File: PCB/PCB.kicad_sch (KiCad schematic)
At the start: 103 parts, among them J1 USB_B_Mini, J2 Screw_Terminal_01x02, J3 Conn_01x03, K1 G6K-2, Q1 IPD50R3K0CE, Q2 2N7002, SW1 SW_Omron_B3FS, U1 STM32F373C8Tx, U2 LIS3MDL, U3 INA848, U4 LM27313XMFX/NOPB, U5 OPA4189xD, U6 THS4561, U7 UCC44273, U8 REF2025AIDDCR, U9 MCP1700-3.3, Y1 8MHz

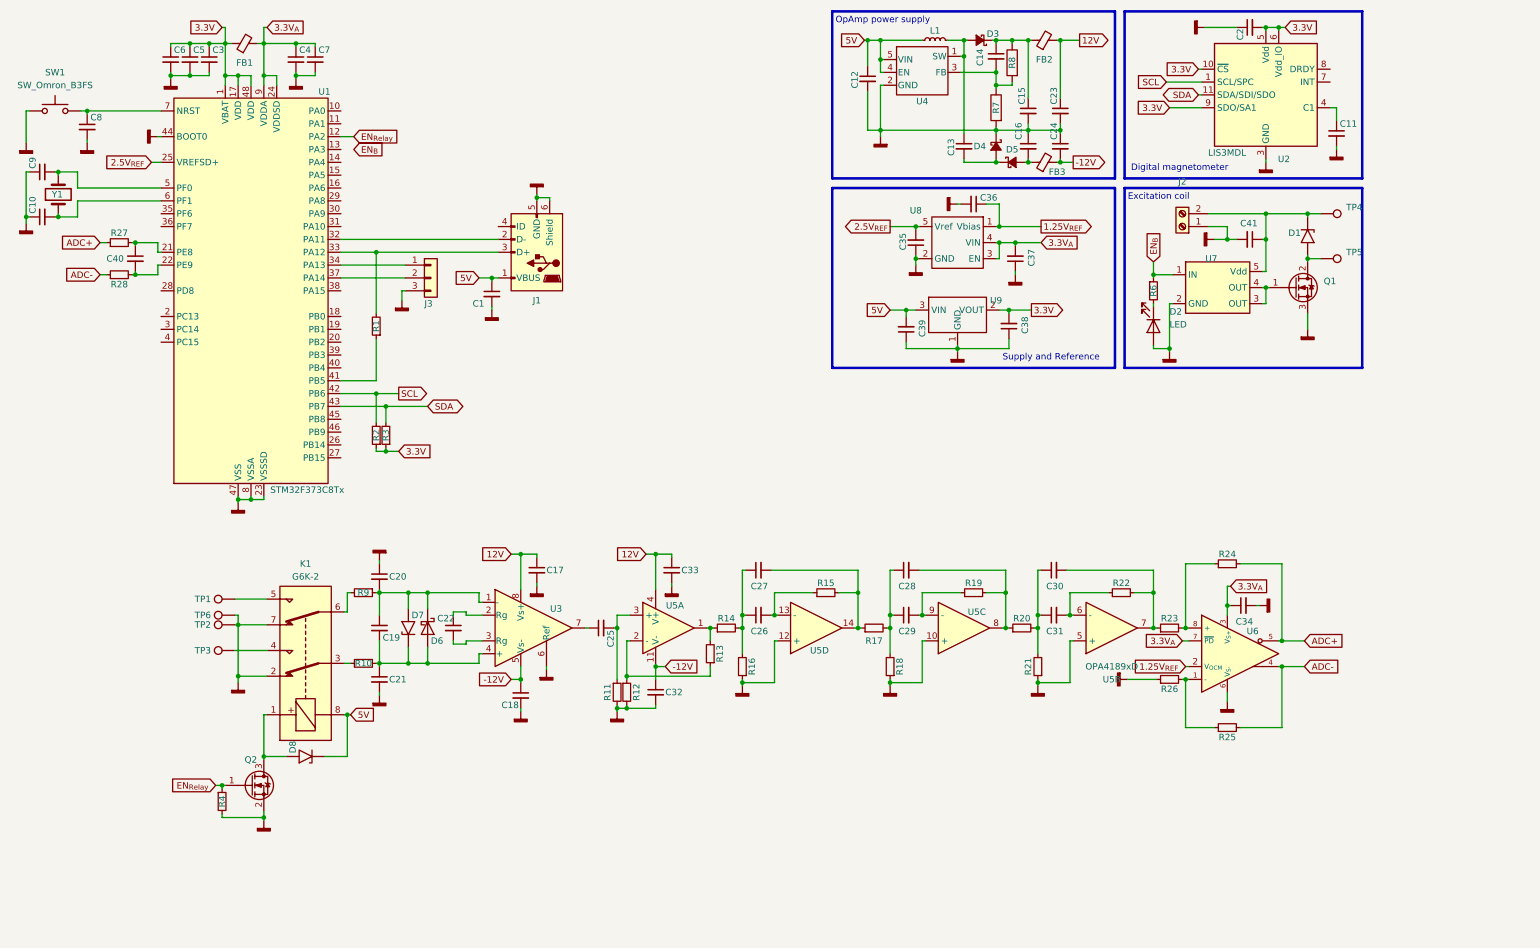
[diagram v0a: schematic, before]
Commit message: Updated
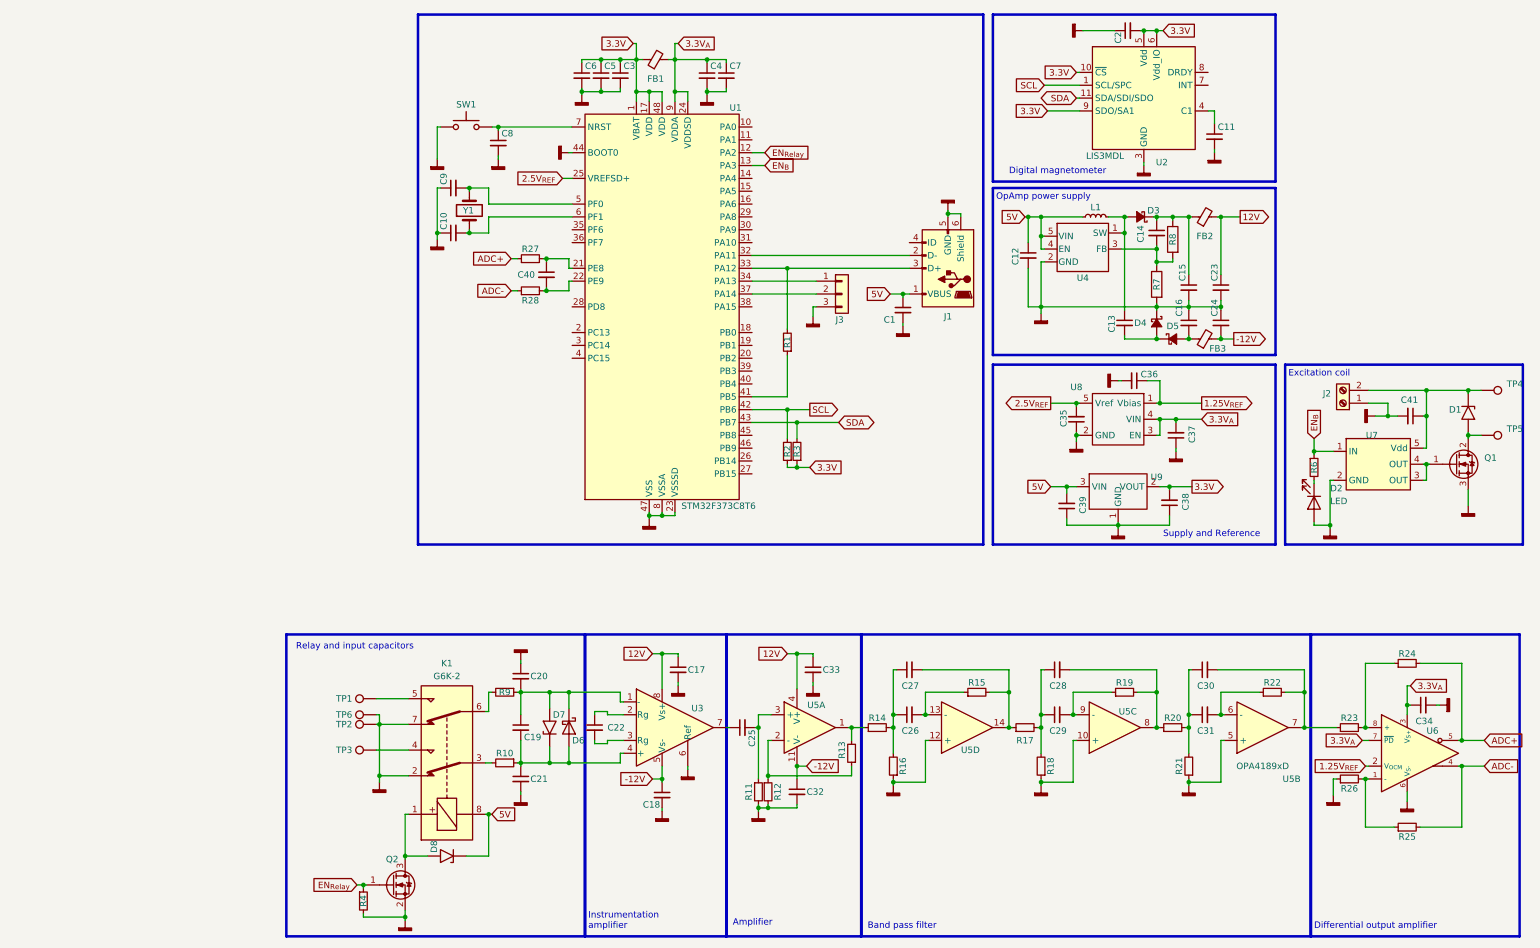
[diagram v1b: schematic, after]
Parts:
- C1: value 100uF -> CC1206MKX5R5BB107; Manufacturer (none) -> Yageo
- C10, C9: value 12pF -> CC0603JRNPO9BN120; Manufacturer (none) -> Yageo
- C11, C2, C3, C4, C6, C7, C8: value 100nF -> CC0603KRX7R9BB104; Manufacturer (none) -> Yageo
- C12, C13, C38, C39: value 100nF -> CC0603KRX7R9BB104; LCSC C14663 -> (none)
- C14: value 120pF -> CC0603JRNPO9BN121; LCSC C107035 -> (none)
- C15, C16, C23, C24: value 1uF -> CC0603KRX7R9BB105; LCSC C559769 -> (none)
- C17, C18, C19, C25, C32, C33, C34: value C_Small -> CC0603KRX7R9BB104; Manufacturer (none) -> Yageo
- C20, C21: value C_Small -> CC0603KRX7R9BB103; Manufacturer (none) -> Ygeo
- C22: value C_Small -> CC0603KRX7R9BB102; Manufacturer (none) -> Yageo
- C26, C27, C28, C29, C30, C31: value C_Small -> CC0603KRX7R9BB103; Manufacturer (none) -> Yageo
- C35, C36, C37, C41: LCSC C14663 -> (none)
- C40: Manufacturer (none) -> Yageo
- C5: value 1uF -> CC0603KRX7R9BB105; Manufacturer (none) -> Yageo
- D3, D4, D5: value SD103AWS-7-F -> SD103AWS; LCSC C154860 -> (none)
- D6: value D_Schottky -> SD101AWS; Manufacturer (none) -> Diodes Incorporated
- D7: value 1.5KExxA -> SD101AWS; Manufacturer (none) -> Diodes Incorporated
- D8: value 1.5KExxA -> SD103AWS; Manufacturer (none) -> Diodes Incorporated
- FB1, FB2, FB3: value FerriteBead_Small -> MPZ1608S601ATD25; Manufacturer (none) -> TDK
- J1: value USB_B_Mini -> 1-1734035-1; Manufacturer (none) -> TE Connectivity
- L1: LCSC C90321 -> (none)
- Q2: Manufacturer (none) -> Diodes Incorporated
- R1: value 1k5 -> RC0603FR-071K5L; Manufacturer (none) -> Yageo
- R10, R28, R9: value R_Small -> RC0603FR-0749R9L; Manufacturer (none) -> Yageo
- R11: value R_Small -> RC0603FR-07100KL; Manufacturer (none) -> Yageo
- R12: value R_Small -> RC0603FR-0710RL; Manufacturer (none) -> Yageo
- R13: value R_Small -> RC0603FR-071KL; Manufacturer (none) -> Yageo
- R14: value R_Small -> RC0603FR-0714K3L; Manufacturer (none) -> Yageo
- R15: value R_Small -> RC0603FR-0745K3L
- R16: value R_Small -> RC0603FR-0715K4L; Manufacturer (none) -> Yageo
- R17: value R_Small -> RC0603FR-075K49L; Manufacturer (none) -> Yageo
- R18: value R_Small -> RC0603FR-076K04L; Manufacturer (none) -> Yageo
- R19: value R_Small -> RC0603FR-0717K4L; Manufacturer (none) -> Yageo
- R2, R3: value 4k7 -> RC0603FR-074K7L; Manufacturer (none) -> Yageo
- R20: value R_Small -> RC0603FR-0713K3L; Manufacturer (none) -> Yageo
- R21, R23, R24, R25, R26, R6: value R_Small -> RC0603FR-075K23L; Manufacturer (none) -> Yageo
- R22: value R_Small -> RC0603FR-07232KL; Manufacturer (none) -> Yageo
- R27: value ~ -> RC0603FR-0749R9L; Manufacturer (none) -> Yageo
- R4: value R_Small -> RC0603FR-074K7L; Manufacturer (none) -> Yageo
- R7: value 15k -> RC0603FR-0715KL; LCSC C114661 -> (none)
- R8: value 150k -> RC0603FR-07150KL; LCSC C114660 -> (none)
- SW1: value SW_Omron_B3FS -> 430182043816; Manufacturer (none) -> Wurth Elektronik
- U1: value STM32F373C8Tx -> STM32F373C8T6; Manufacturer (none) -> STMicroelectronics
- U2, U3, U5, U6, U7: Manufacturer (none) -> Texas Instruments
- U4: LCSC C341750 -> (none)
- U8: LCSC C962078 -> (none)
- U9: value MCP1700-3.3 -> TPS7A0533PDBZR; LCSC C2877921 -> (none)
- Y1: value 8MHz -> 830003151; Manufacturer (none) -> Wurth Elektronik
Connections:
- net EN_{B}: now also U1.13 (PA3)
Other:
- note added: "Amplifier"
- note added: "Band pass filter"
- note added: "Differential output amplifier"
- note added: "Instrumentation amplifier"
- note added: "Relay and input capacitors"
- moved on the sheet: C1, C10, C11, C12, C13, C14, C15, C16, C17, C18, C19, C2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
